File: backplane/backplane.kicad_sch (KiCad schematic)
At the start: 29 parts, among them J101 DIN41612_02x16_AC_EvenPins, J102 DIN41612_02x16_AC_EvenPins, J103 DIN41612_02x16_AC_EvenPins, J104 DIN41612_02x16_AC_EvenPins, J105 DIN41612_02x16_AC_EvenPins, J106 DIN41612_02x16_AC_EvenPins, J107 DIN41612_02x16_AC_EvenPins, J108 DIN41612_02x16_AC_EvenPins, J109 Conn_01x03, J110 Conn_01x03, J111 Conn_01x01, J112 Conn_01x01

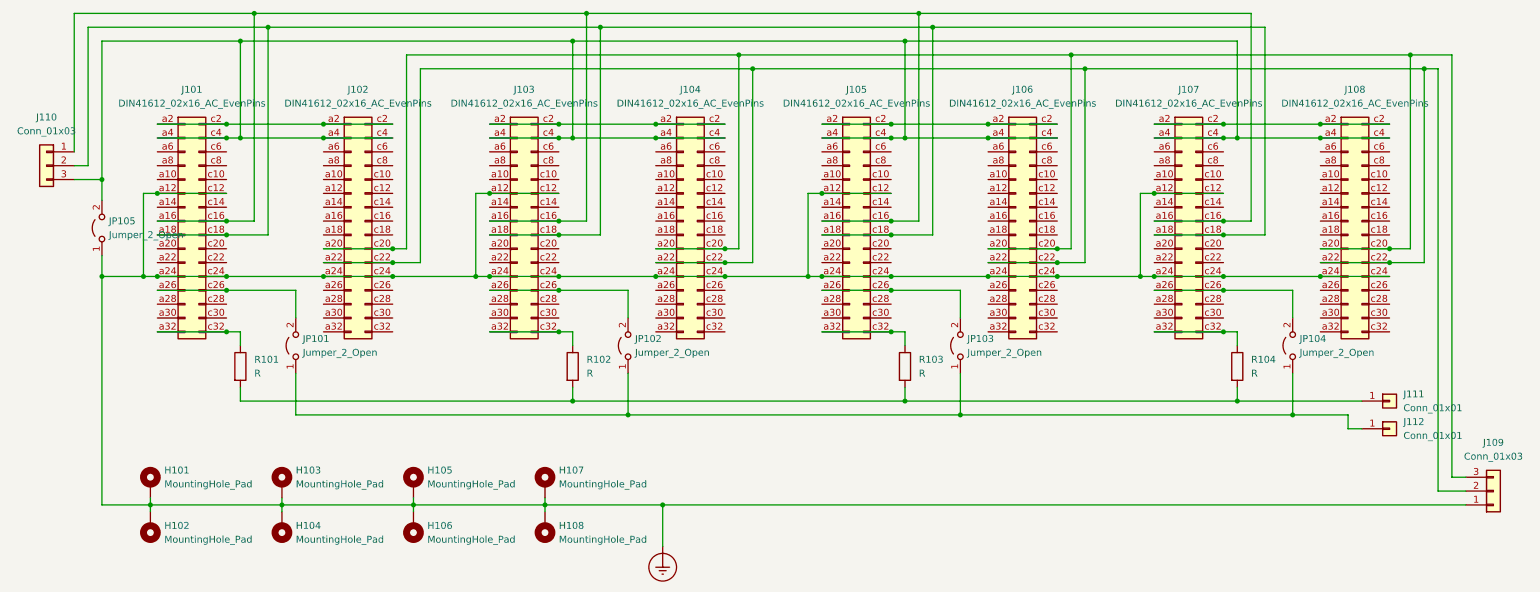
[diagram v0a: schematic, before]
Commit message: Update backplane.kicad_sch
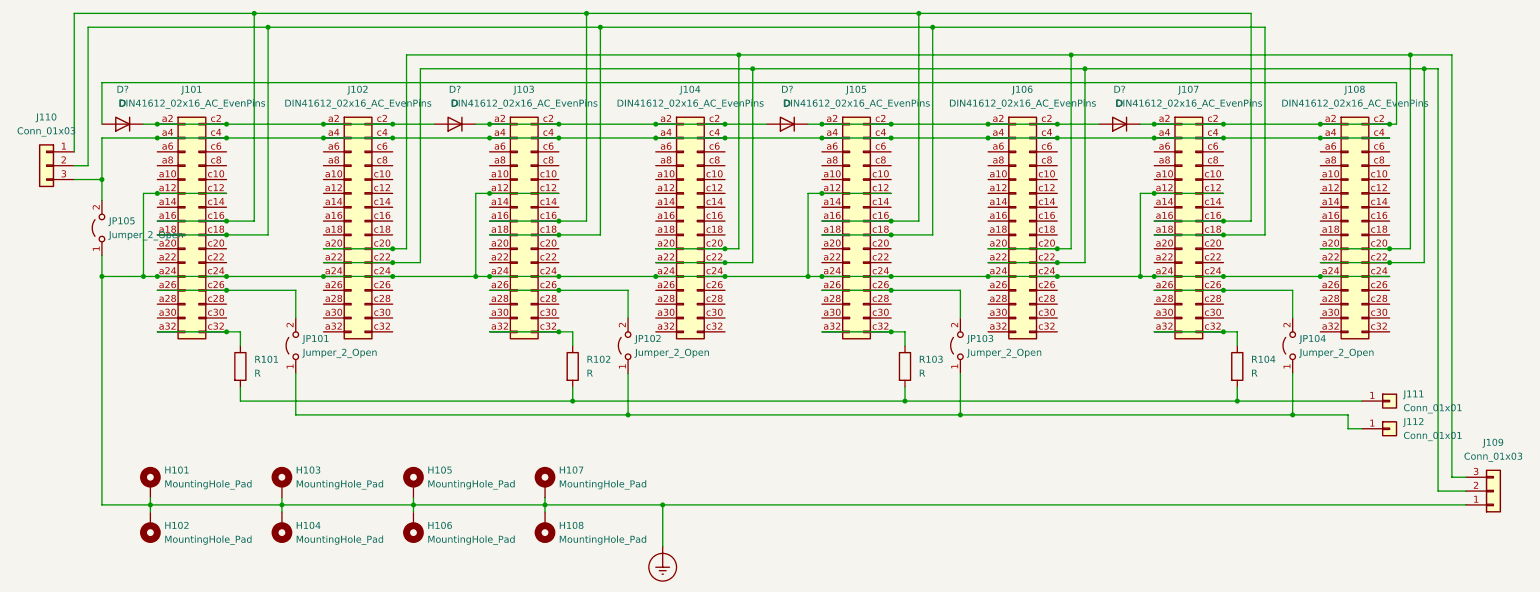
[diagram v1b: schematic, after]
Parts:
- added D? (x4): D, Diode_THT:D_A-405_P12.70mm_Horizontal, symbol Device:D
- JP105: footprint Jumper:SolderJumper-2_P1.3mm_Open_RoundedPad1.0x1.5mm -> Jumper:SolderJumper-2_P1.3mm_Bridged_RoundedPad1.0x1.5mm
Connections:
- net at J107.a2 (Pin_a2), J107.c2 (Pin_c2), J108.a2 (Pin_a2)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: now also D?.1 (K), D?.2 (A)
- net at J105.a2 (Pin_a2), J105.c2 (Pin_c2), J106.a2 (Pin_a2)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: now also D?.1 (K), D?.2 (A)
- net at J103.a2 (Pin_a2), J103.c2 (Pin_c2), J104.a2 (Pin_a2)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: now also D?.1 (K), D?.2 (A)
- net at J101.a2 (Pin_a2), J101.c2 (Pin_c2), J102.a2 (Pin_a2)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: now also D?.1 (K), D?.2 (A)
